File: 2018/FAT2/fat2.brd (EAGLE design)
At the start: 120 x 80 mm, 32 parts, among them Q1 BUZ11BV, Q2 BUZ11BV

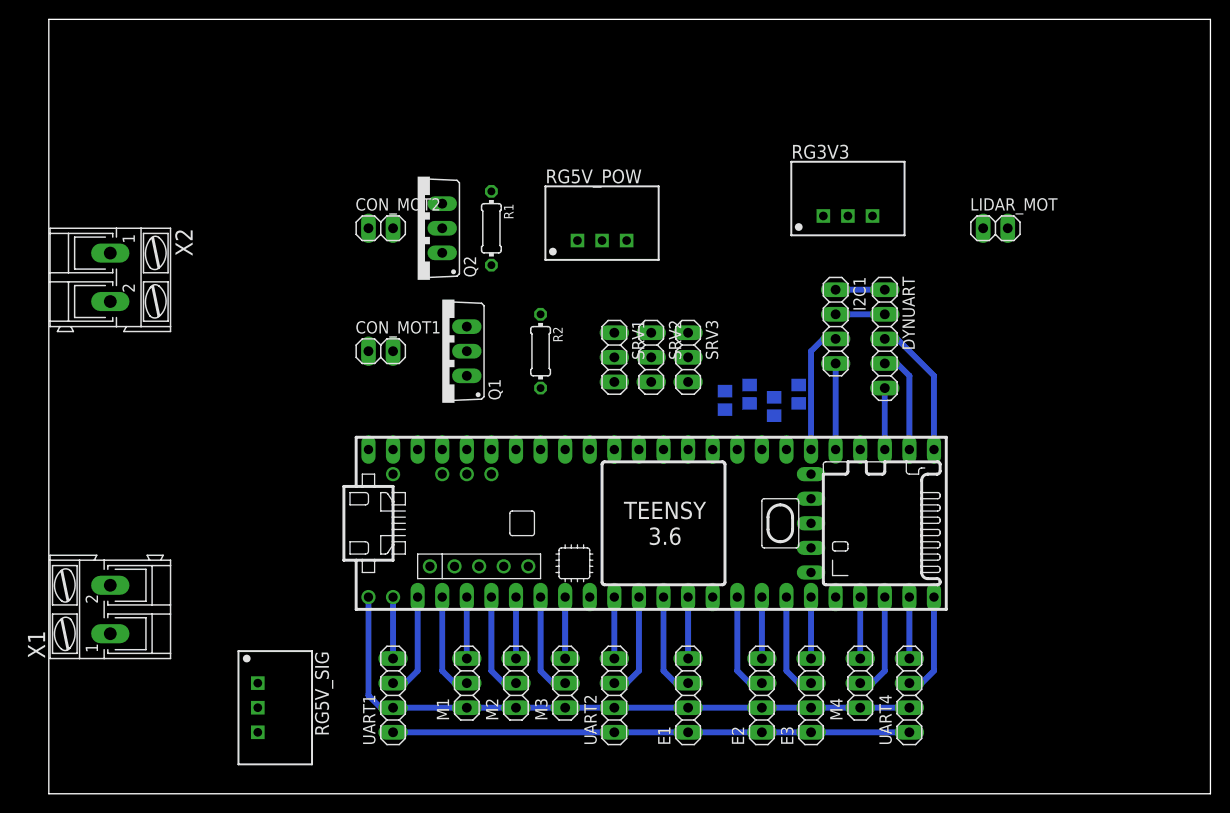
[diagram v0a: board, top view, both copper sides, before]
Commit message: [FAT V2] Finish board.
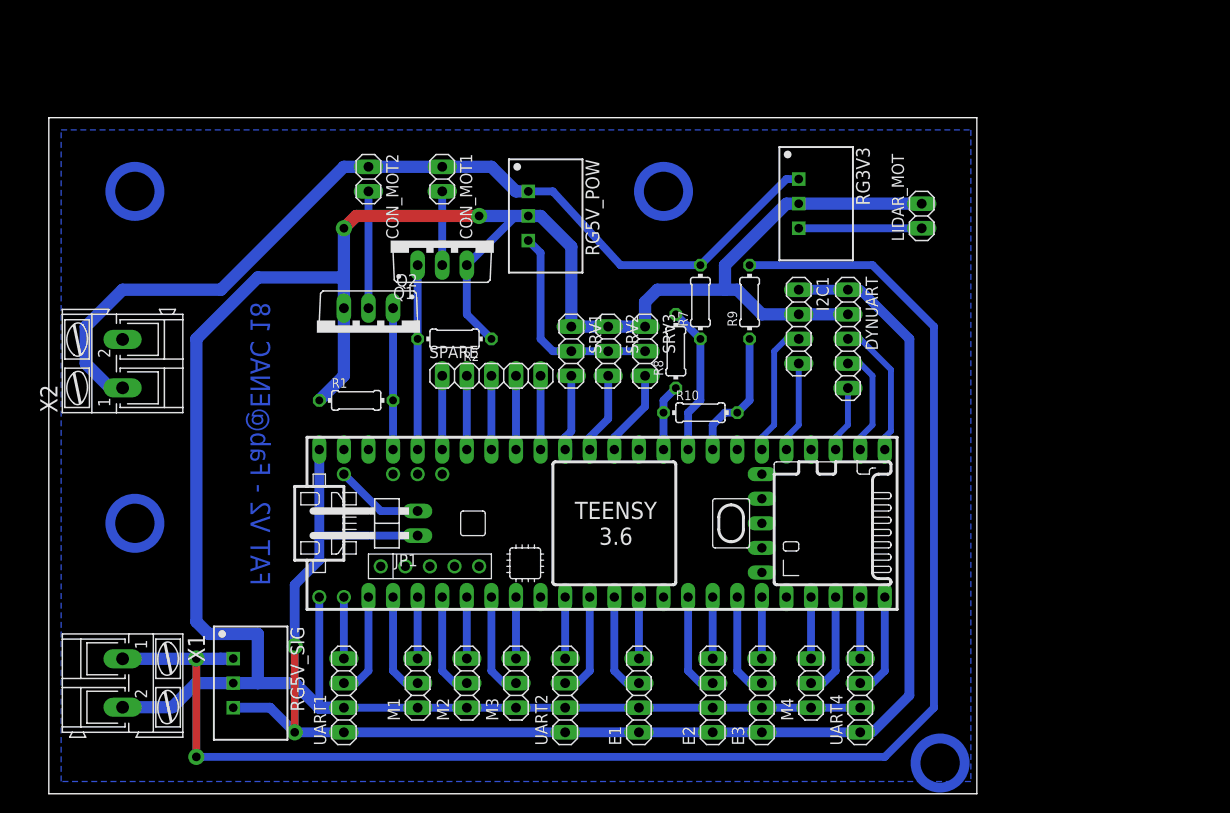
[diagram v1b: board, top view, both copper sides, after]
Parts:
- removed R3, R4, R5, R6: (no value), rcl:R0805
- added JP1: (no value), pinhead:1X02/90
- added R10, R7, R8, R9: 10k, rcl:0204/7
- added SPARE: (no value), pinhead:1X05
- moved R1 22.6 mm to (31.8, 40.6), turned to 0 degrees
- moved CON_MOT1 18.9 mm to (40.6, 63.5), turned to 270 degrees
- moved Q2 11.9 mm to (33.0, 47.6), turned to 180 degrees
- moved Q1 11.4 mm to (40.6, 57.1), turned to 0 degrees
- moved R2 8.98 mm to (41.9, 47.0), turned to 180 degrees
- moved X2 8.98 mm to (7.62, 44.5), turned to 90 degrees
- moved RG5V_POW 8.03 mm to (49.5, 59.7), turned to 270 degrees
- moved LIDAR_MOT 7.73 mm to (90.2, 59.7), turned to 90 degrees
- moved X1 7.73 mm to (7.62, 11.4), turned to 270 degrees
- moved RG3V3 5.24 mm to (77.5, 61.0), turned to 270 degrees
- moved CON_MOT2 5.24 mm to (33.0, 63.5), turned to 270 degrees
- moved UART4 5.08 mm to (83.8, 10.2)
- moved E1 5.08 mm to (61.0, 10.2)
- moved M3 5.08 mm to (48.3, 11.4)
- moved UART1 5.08 mm to (30.5, 10.2)
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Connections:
- new net GND2: R10.1, R8.1, U$1.GND2
- new net N$1: SPARE.5, U$1.17/A3
- new net N$2: SPARE.4, U$1.18/A4/SDA
- new net N$4: SPARE.3, U$1.19/A5/SCL
- new net N$8: SPARE.1, U$1.21/A7
- net 12V_POW: now also R7.2; no longer R4.2
- net 12V_SIG: now also R9.2; no longer R5.2
- net 5V_SIG: now also JP1.1, U$1.VIN
- net GND: now also Q1.S, Q2.S, R1.1, R2.1; no longer R3.1, R6.1
- net N$6: now also SPARE.2, U$1.20/A6; no longer U$1.17/A3
- net N$7: now also JP1.2, U$1.VUSB; no longer Q1.S, Q2.S, R1.1, R2.1
- net POW_LEVEL: now also R7.1, R8.2; no longer R3.2, R4.1
- net SIG_LEVEL: now also R10.2, R9.1; no longer R5.1, R6.2
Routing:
- net GND: track 71.6 -> 276.5 mm, vias 0 -> 2
- net 12V_SIG: track 0.00 -> 161.0 mm, vias 0 -> 2
- net 5V_SIG: track 59.7 -> 164.5 mm, vias 0 -> 2
- net 12V_POW: track 0.00 -> 97.2 mm
- net 5V_POW: track 0.00 -> 22.0 mm
- net MOT1: track 0.00 -> 19.0 mm
- net POW_LEVEL: track 0.00 -> 15.5 mm
- net MOT2: track 0.00 -> 14.6 mm
- net SIG_LEVEL: track 0.00 -> 13.8 mm
- net 3V3: track 0.00 -> 12.7 mm
- net N$5: track 0.00 -> 12.1 mm
- net N$7: track 0.00 -> 9.20 mm
- net SERVO3: track 0.00 -> 8.94 mm
- net SERVO2: track 0.00 -> 8.41 mm
- net SERVO1: track 0.00 -> 7.88 mm
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- added copper zone on layer 16, net GND
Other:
- board size 120 x 80 mm -> 95.9 x 69.8 mm
- board text added: "FAT V2 - Fab@ENAC 18"
